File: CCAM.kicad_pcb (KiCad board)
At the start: 2 copper layers, 74.3 x 64.8 mm, 59 parts, among them J1 32XL, J10 OUTL, J11 OUTR, J2 MCDL, J3 FML, J4 PSG, J5 FMR, J6 MCDR, J7 32XR, J8 5Vin, J9 GNDin, Q1 MMBT3904, Q2 MMBT3904, Q3 MMBT3904, Q4 MMBT3904, U1 RC4558

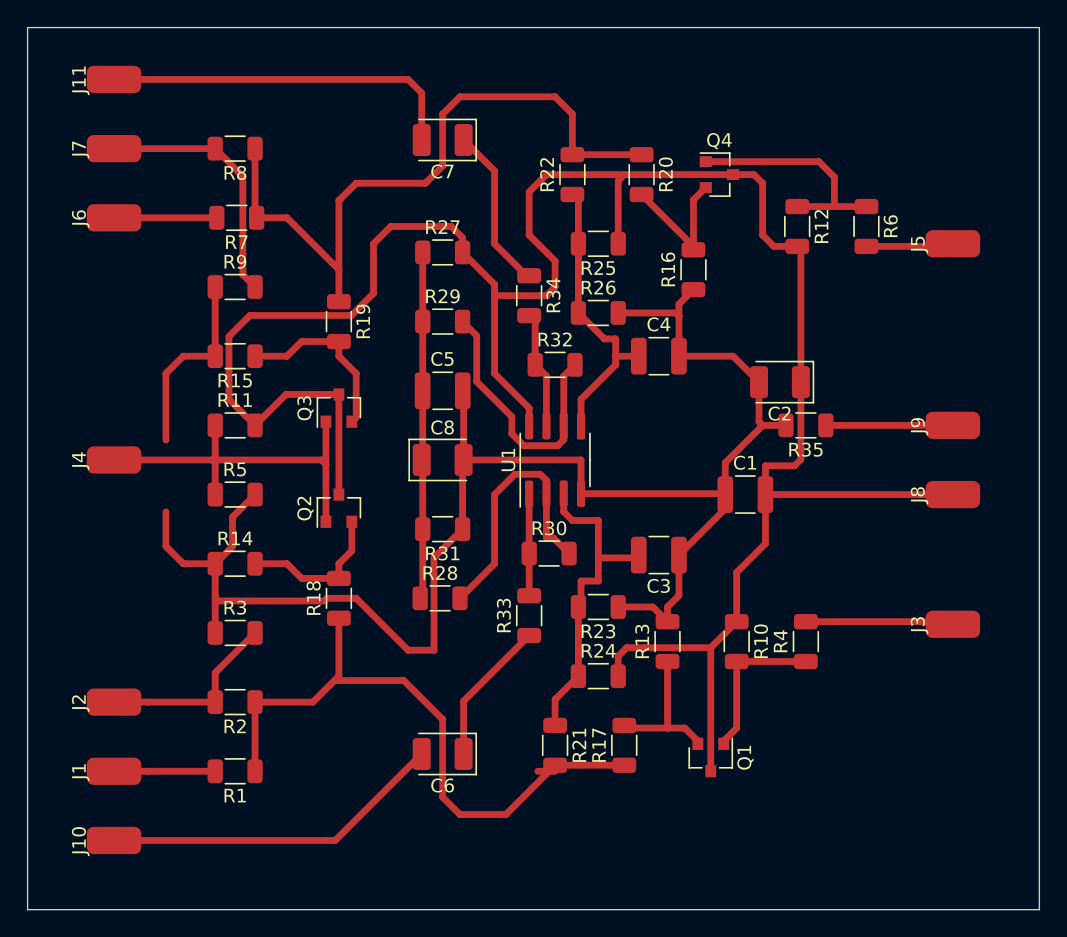
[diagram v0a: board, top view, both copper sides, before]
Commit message: Board optimization
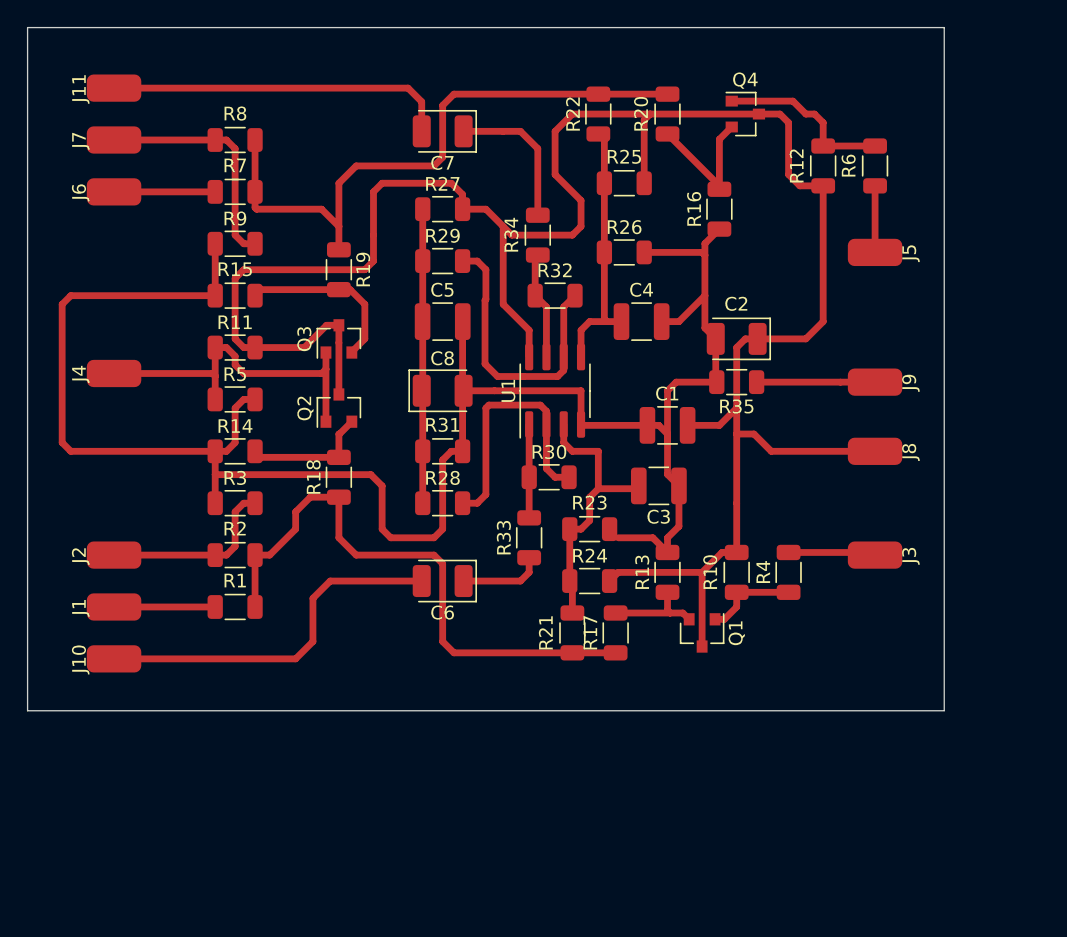
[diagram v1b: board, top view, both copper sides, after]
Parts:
- moved J10 13.3 mm to (17.8, 81.9)
- moved C6 12.7 mm to (41.9, 76.2)
- moved J1 12.1 mm to (17.8, 78.1)
- moved R1 12.1 mm to (26.7, 78.1)
- moved J2 10.8 mm to (17.8, 74.3)
- moved R2 10.8 mm to (26.7, 74.3)
- moved R3 9.53 mm to (26.7, 70.5)
- moved Q1 9.17 mm to (61.0, 80.0)
- moved R18 8.89 mm to (34.3, 68.6)
- moved R21 8.35 mm to (51.4, 80.0)
- moved R17 8.28 mm to (54.6, 80.0)
- moved R14 8.26 mm to (26.7, 66.7)
- moved C1 7.65 mm to (58.4, 64.8)
- moved J3 7.65 mm to (73.7, 74.3), turned to 270 degrees
- moved Q2 7.35 mm to (34.3, 63.5)
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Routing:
- net GND: track 134.5 -> 143.4 mm
- net Net-(R19-Pad1): track 51.3 -> 45.7 mm
- net Net-(R1-Pad1): track 47.7 -> 42.6 mm
- net +5V: track 167.9 -> 162.9 mm
- net Net-(C6-Pad1): track 10.7 -> 6.15 mm
- net Net-(Q1-Pad1): track 11.3 -> 6.85 mm
- net Net-(J3-Pad1): track 10.9 -> 6.43 mm
- net Net-(Q4-Pad1): track 17.2 -> 12.9 mm
- net Net-(C5-Pad1): track 25.5 -> 21.6 mm
- net Net-(C3-Pad2): track 24.3 -> 20.5 mm
- net Net-(Q1-Pad2): track 11.1 -> 7.38 mm
- net Net-(J4-Pad1): track 28.4 -> 25.8 mm
- net Net-(C4-Pad1): track 21.6 -> 19.2 mm
- net Net-(Q2-Pad2): track 11.2 -> 9.38 mm
- net Net-(R29-Pad2): track 19.9 -> 21.5 mm
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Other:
- board size 74.3 x 64.8 mm -> 67.3 x 50.2 mm
